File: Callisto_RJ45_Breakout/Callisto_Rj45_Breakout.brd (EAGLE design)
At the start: 50 x 60 mm, 11 parts, among them J1 RJ45_TH_VERT, J11 2-pos, J4 4-pos, SW1 PTS810SJG250SMTRLFS, SW4 PTS810SJG250SMTRLFS

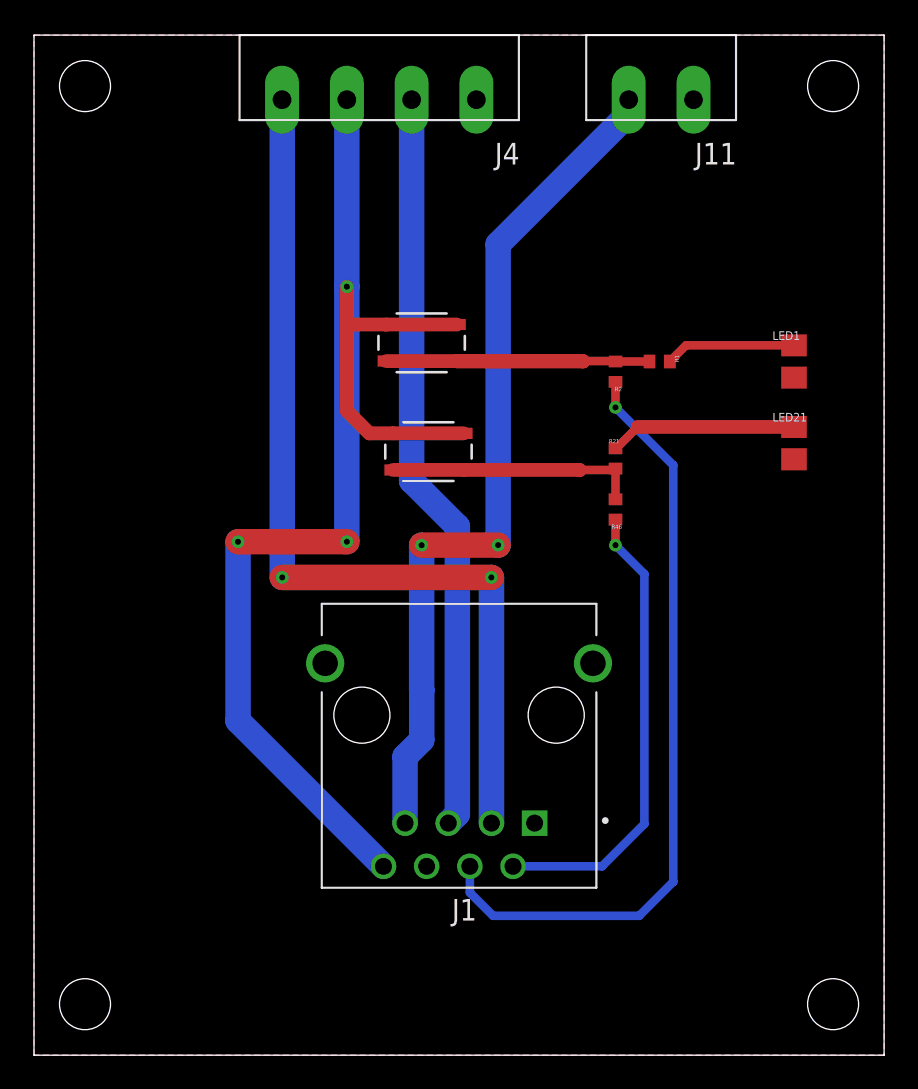
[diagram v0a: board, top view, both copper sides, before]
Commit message: Updated boards
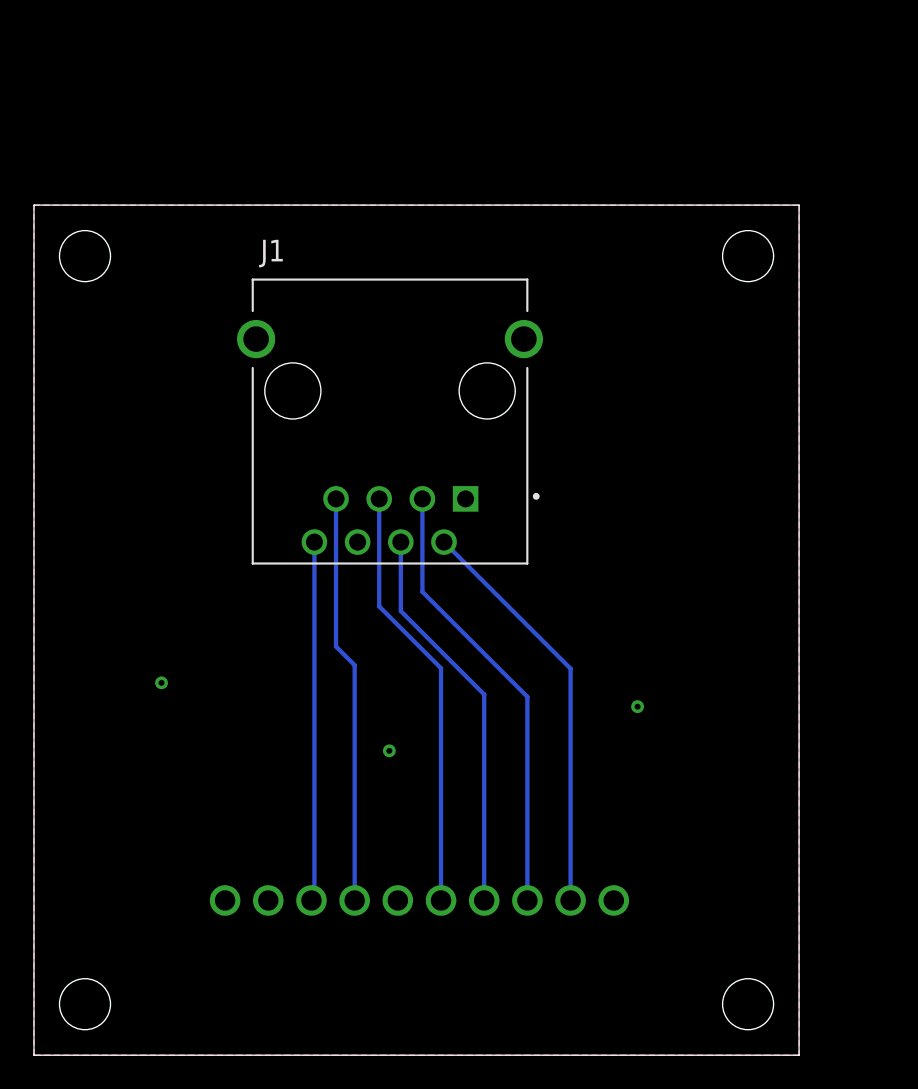
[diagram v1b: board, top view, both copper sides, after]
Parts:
- removed J11: 2-pos, 3D_MIG_Controller:2_3.81MM_PITCH
- removed J4: 4-pos, 3D_MIG_Controller:1X4_3.81MM_PITCH
- removed LED1, LED21: Green, 3D_MIG_Controller:0805
- removed R1, R21: 470R, 3D_MIG_Controller:0402
- removed R2, R46: 470, 3D_MIG_Controller:0402
- removed SW1, SW4: PTS810SJG250SMTRLFS, 3D_MIG_Controller:PTS810
- added U$1: 1_X_10_HEADER_GENERIC_.1INCH, 3D_MIG_Controller:HEADER_1_X_10_.1_INCH
- moved J1 19.5 mm to (20.9, 39.1)
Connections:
- removed net N$103: R21.P$2, R46.P$2, SW4.3, SW4.4
- removed net N$2: R1.P$2, R2.P$2, SW1.3, SW1.4
- removed net N$37: J1.4, R2.P$1
- removed net N$41: LED21.1, R21.P$1
- net GND: now also U$1.P$1, U$1.P$10, U$1.P$6, U$1.P$9; no longer J11.P$1, J4.P$1, LED1.2, LED21.2
- net IO_SIGNAL: now also U$1.P$2; no longer R46.P$1
- net N$1: now also J1.4, U$1.P$4; no longer LED1.1, R1.P$1
- net VDD: now also U$1.P$5; no longer J4.P$2
- net VDD-12: now also U$1.P$7; no longer J11.P$2
- net VDD12: now also U$1.P$3; no longer J4.P$4
- net VDD5: now also U$1.P$8; no longer J4.P$3, SW1.1, SW1.2, SW4.1, SW4.2
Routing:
- net VDD5: track 76.2 -> 21.2 mm, vias 3 -> 0
- net N$37: track 45.7 -> 0.00 mm, vias 1 -> 0
- net VDD12: track 55.1 -> 26.2 mm, vias 2 -> 0
- net VDD-12: track 50.6 -> 24.1 mm, vias 2 -> 0
- net N$2: track 22.9 -> 0.00 mm
- net VDD: track 43.9 -> 25.1 mm
- net N$1: track 7.69 -> 23.1 mm
- net N$103: track 14.9 -> 0.00 mm
- net N$41: track 11.0 -> 0.00 mm
- net IO_SIGNAL: track 27.4 -> 24.2 mm, vias 1 -> 0
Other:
- board size 50 x 60 mm -> 45 x 50 mm
